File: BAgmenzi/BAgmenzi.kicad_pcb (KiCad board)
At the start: 6 copper layers, 64.8 x 44.8 mm, 155 parts, among them IC1 TPL0501-100RSER, J1 Conn_01x07, J2 DF52-2S-0.8H(21), J3 USB3076-30-A, J5 3220-10-0100-00, Q1 NX7002BKMBYL, U1 MSP430FR5043IRGCT, U10 PESD1USB30, U11 MAX77654BENV+T, U13 TPS7A2033DBVDQN, U2 AD8338ACPZ-R7, U3 OPA836IDBVT, U4 OPA836IDBVT, U5 polyCMUT, U6 DNP, U7 LT3463AEDD#PBF, U8 TPS22916CYFPR, U9 MAXM86161EFD_T, X1 FY0800018, X2 ABS07-32.768KHZ-9-T, Y1 AWSCR-8.00CV-T

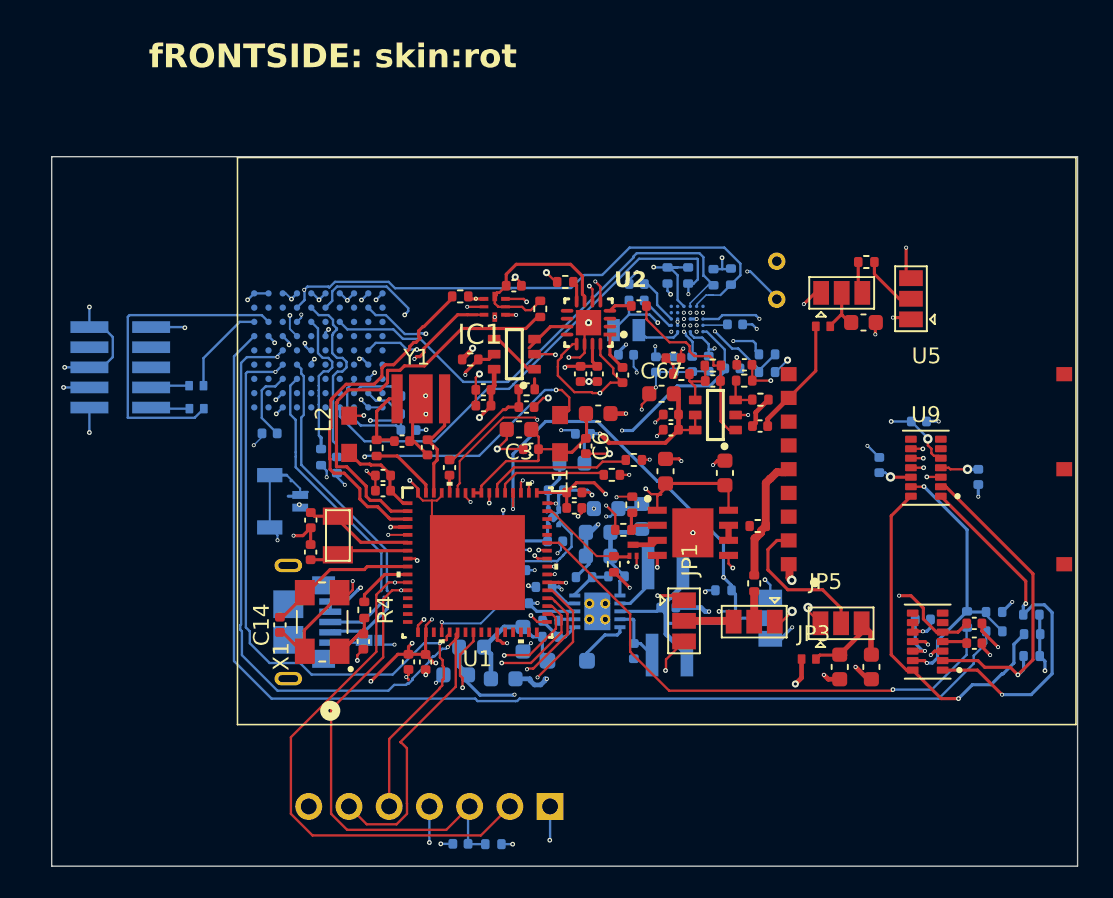
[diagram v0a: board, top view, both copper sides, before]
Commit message: edge cuts
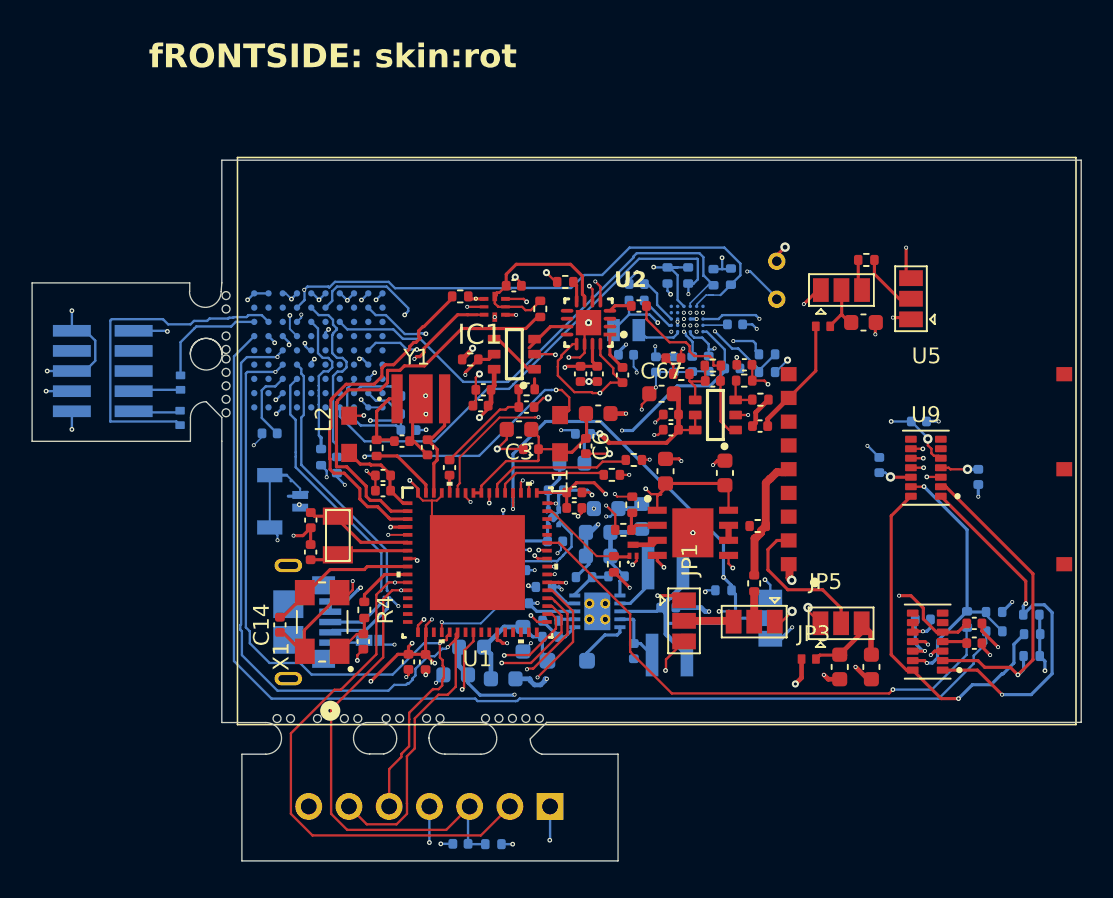
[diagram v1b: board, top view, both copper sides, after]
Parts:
- added REF**: MouseBite-Part_2.0x2.0mm_inset_D0.5mm_P0.85mm_5h, Panelization:MouseBite-Part_2.0x2.0mm_inset_D0.5mm_P0.85mm_5h, F.Cu at (118.3, 103.5)
- added REF**: MouseBite-Part_2.0x2.0mm_inset_D0.5mm_P0.85mm_4h_Trace, Panelization:MouseBite-Part_2.0x2.0mm_inset_D0.5mm_P0.85mm_4h_Trace, F.Cu at (130.4, 124.8)
- added REF**: MouseBite-Part_2.0x2.0mm_inset_D0.5mm_P0.85mm_4h_Trace, Panelization:MouseBite-Part_2.0x2.0mm_inset_D0.5mm_P0.85mm_4h_Trace, F.Cu at (118.3, 99.5)
- added REF**: MouseBite-Part_2.0x2.0mm_inset_D0.5mm_P0.85mm_5h, Panelization:MouseBite-Part_2.0x2.0mm_inset_D0.5mm_P0.85mm_5h, F.Cu at (136.6, 124.8)
- added REF**: MouseBite-Part_2.0x4.5mm_inset_D0.5mm_P0.85mm_5h_Trace, Panelization:MouseBite-Part_2.0x4.5mm_inset_D0.5mm_P0.85mm_5h_Trace, F.Cu at (124.3, 124.8)
- moved R45 1.20 mm to (115.6, 105.5), turned to -90 degrees
- moved J5 1.13 mm to (110.8, 102.6)
- moved R46 1.01 mm to (115.7, 103.3), turned to 90 degrees
- moved JP4 0.18 mm to (157.4, 97.5)
- moved C21 0.18 mm to (134.6, 104.8)
- moved R41 0.13 mm to (159.0, 95.5)
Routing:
- net GND: track 151.9 -> 154.2 mm, vias 108 -> 110
- net Net-(X1-IN/OUT): track 5.04 -> 3.03 mm
- net SWCLK: track 5.89 -> 7.28 mm
- net /RX/VGA_REF: track 25.0 -> 23.6 mm
- net nRST: track 46.4 -> 47.6 mm
- net SWDIO: track 20.5 -> 21.5 mm
- net Net-(J5-Pad2): track 3.30 -> 3.85 mm
- net Net-(J5-Pad4): track 2.44 -> 3.00 mm
- net DVDD_3.3: track 74.1 -> 73.6 mm
- added copper zone on In2.Cu, net GND
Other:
- board size 64.8 x 44.8 mm -> 66.3 x 44.2 mm
